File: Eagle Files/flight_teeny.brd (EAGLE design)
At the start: 55.8 x 39.8 mm, 21 parts, among them M4 WIRELESS-NRF24L01, Q1 SI2302, Q2 SI2302, Q3 SI2302, Q5 SI2302, U2 GY-521MPU6050

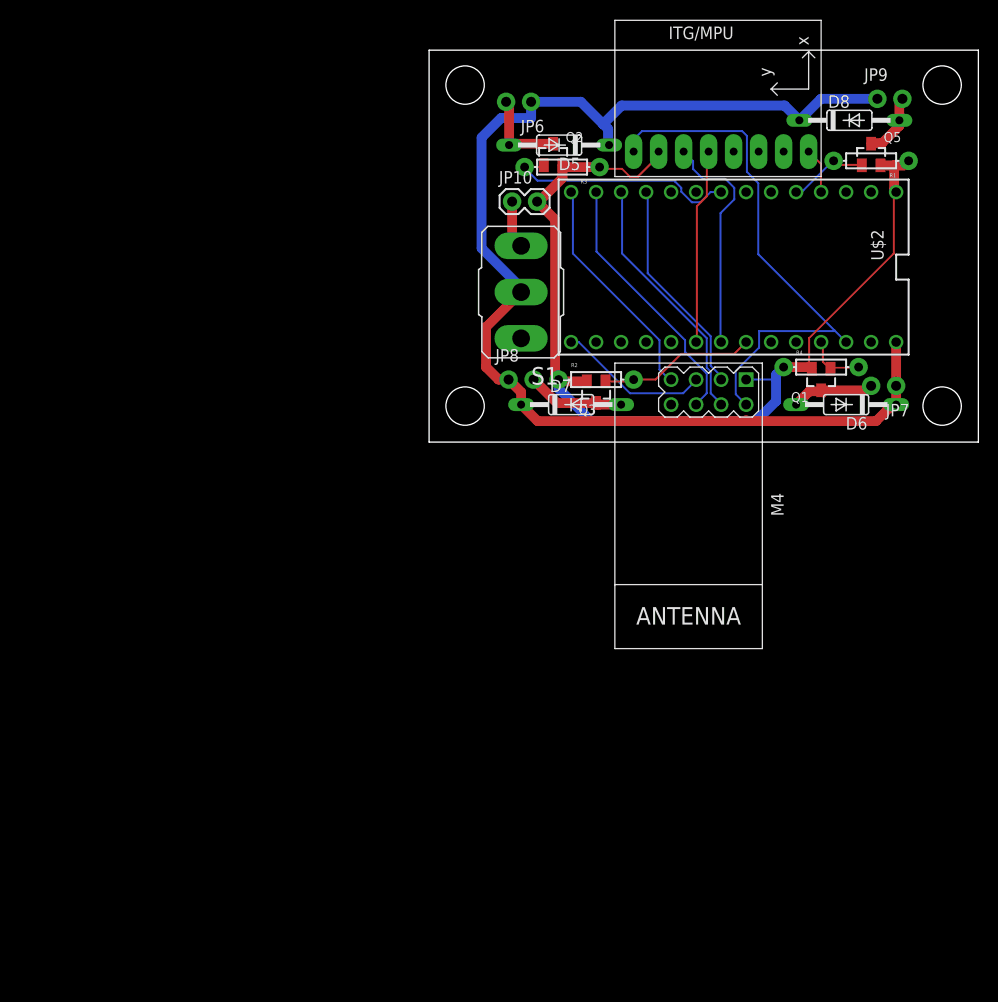
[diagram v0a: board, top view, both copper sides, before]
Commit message: PCB Shape Added
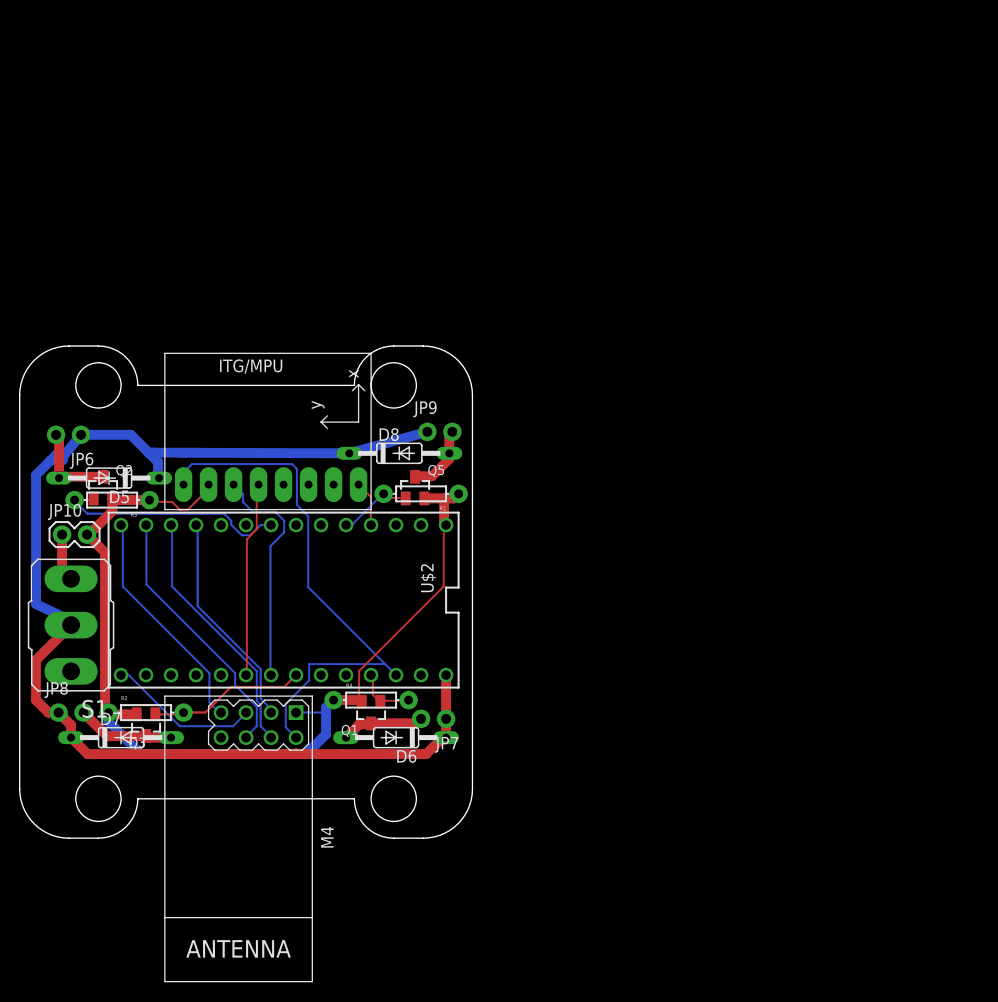
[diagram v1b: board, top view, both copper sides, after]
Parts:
- moved Q5 57.4 mm to (17.2, 10.6)
- moved JP7 56.9 mm to (20.3, -12.9)
- moved M4 56.9 mm to (-1.27, -24.9)
- moved D5 56.9 mm to (-13.9, 11.6)
- moved D6 56.9 mm to (15.2, -14.8)
- moved D7 56.9 mm to (-12.7, -14.8)
- moved D8 56.9 mm to (15.6, 14.1)
- moved JP10 56.9 mm to (-18.7, 5.84)
- moved JP6 56.9 mm to (-16.8, 16.0)
- moved JP8 56.9 mm to (-19.1, -12.2)
- moved Q1 56.9 mm to (12.7, -12.2)
- moved Q2 56.9 mm to (-14.5, 10.6)
- moved Q3 56.9 mm to (-10.2, -13.5)
- moved R1 56.9 mm to (17.8, 9.98)
- moved R2 56.9 mm to (-10.2, -12.2)
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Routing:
- net P_IN: track 133.3 -> 132.0 mm
- net N$15: track 6.49 -> 7.10 mm
- net GND: track 105.2 -> 105.8 mm
- net PWM1: track 8.17 -> 7.56 mm
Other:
- board size 55.8 x 39.8 mm -> 46 x 50 mm
